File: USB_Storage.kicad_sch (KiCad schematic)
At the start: 26 parts, among them J1 USB_A, U1 USBLC6-2SC6, U2 AP2112K-3.3, U3 GL3224-ONY, U4 AP2112K-1.2, Y1 25MHz

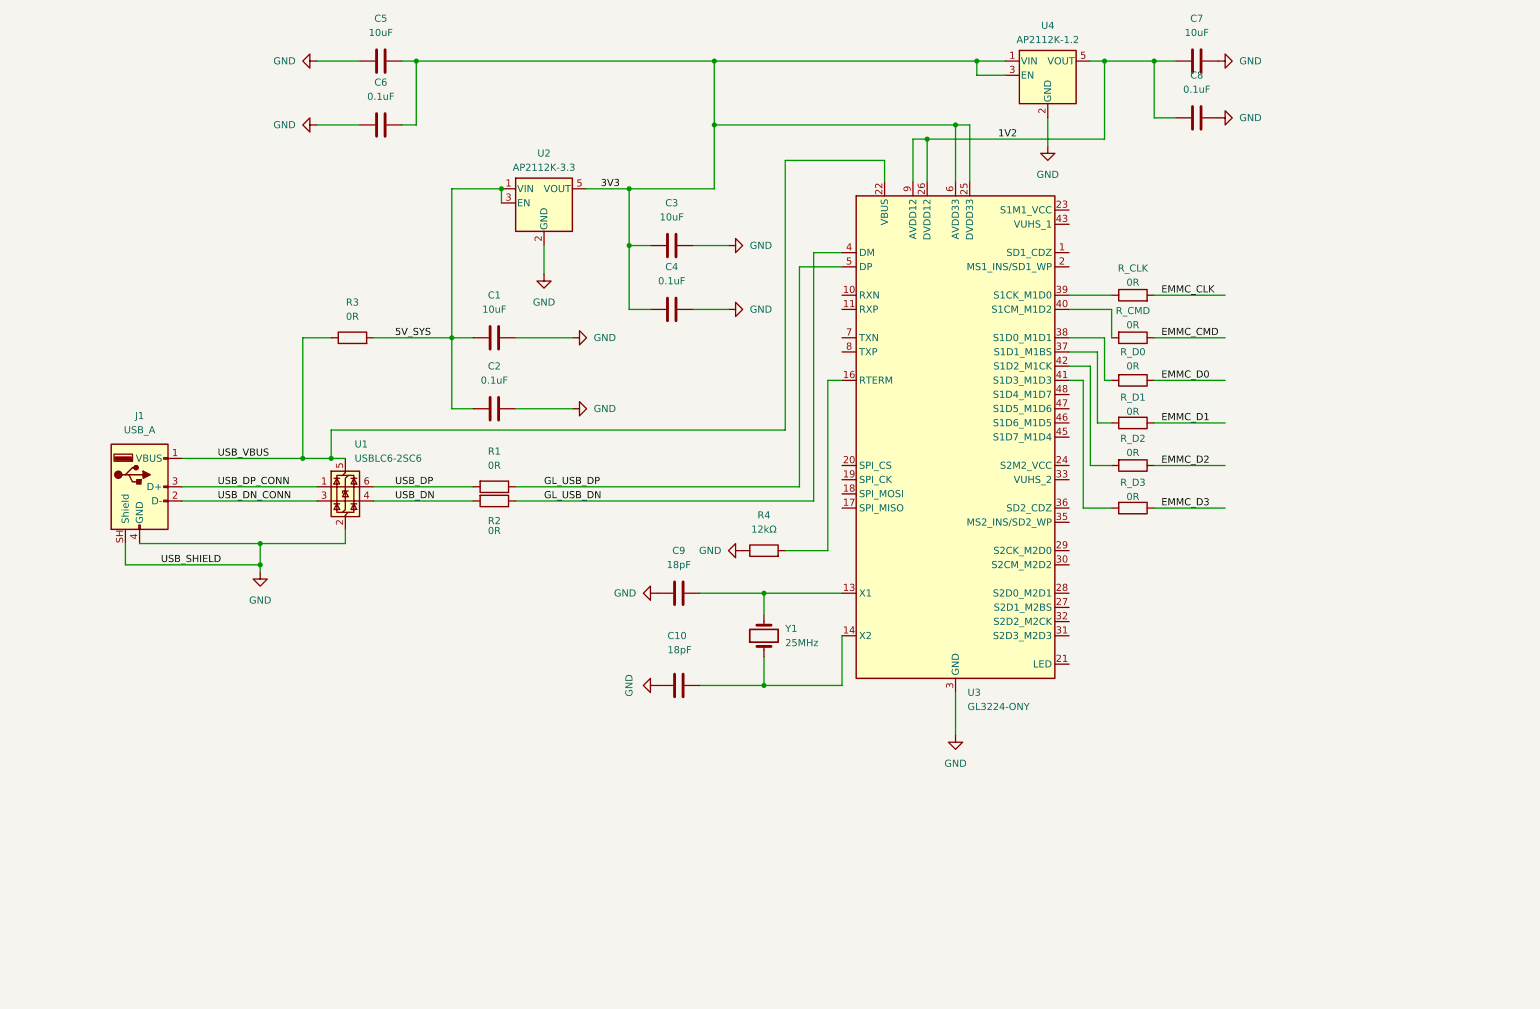
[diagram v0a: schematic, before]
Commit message: 回路図を更新しました
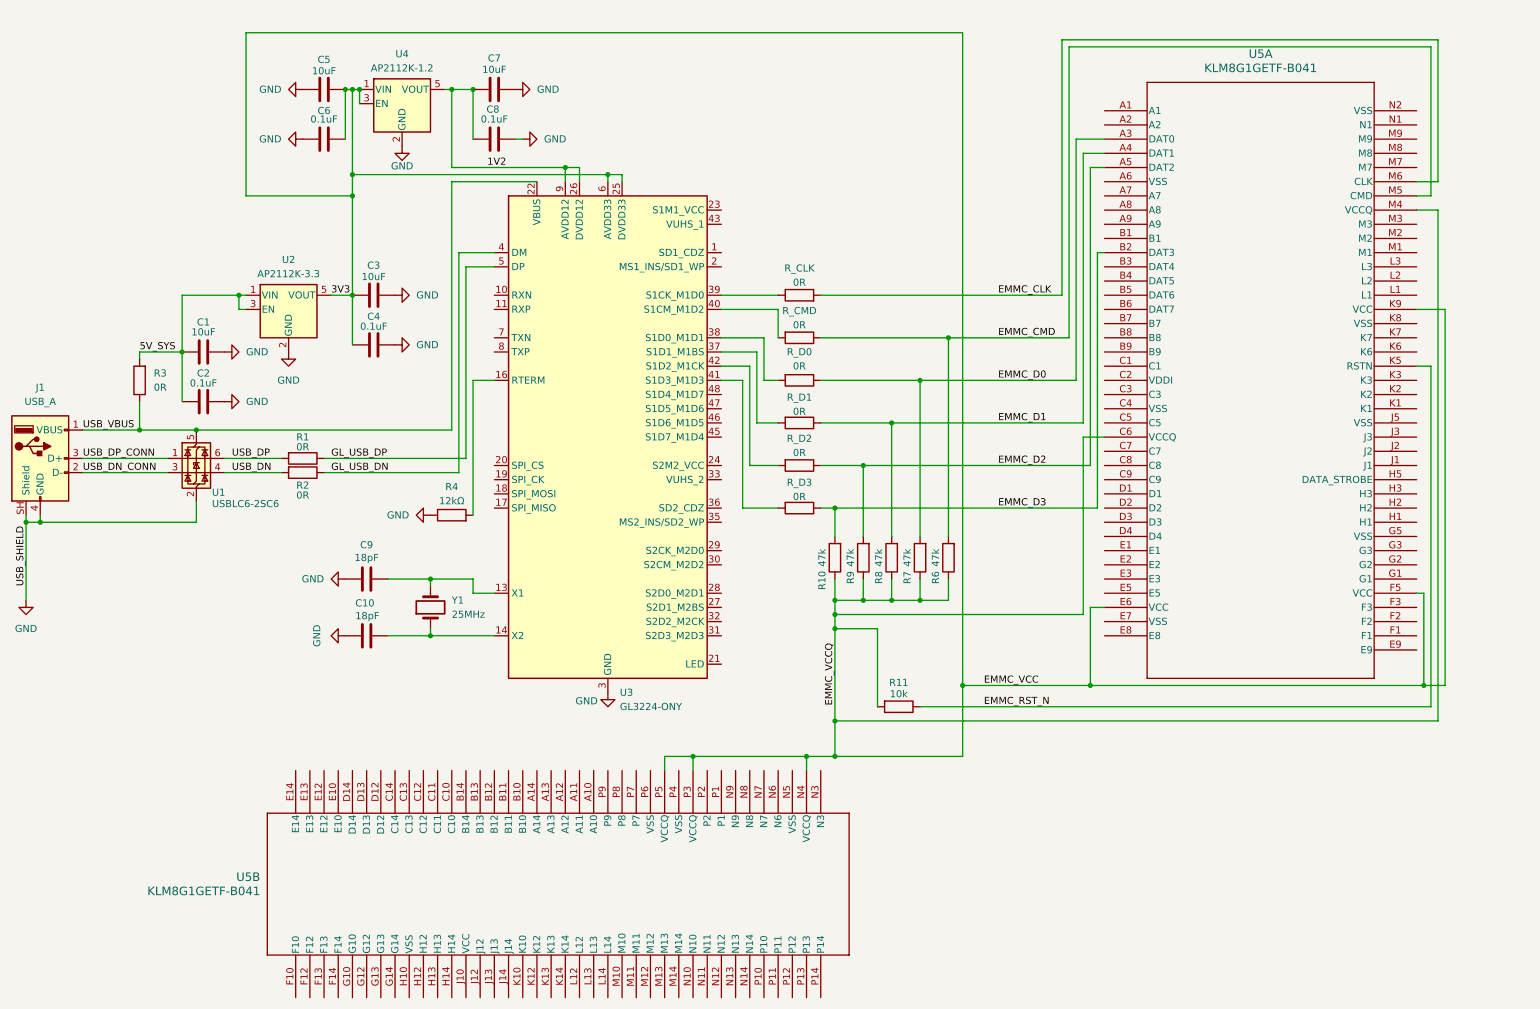
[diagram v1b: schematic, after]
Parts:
- added R10, R6, R7, R8, R9: 47k, symbol Device:R
- added R11: 10k, symbol Device:R
- added U5: KLM8G1GETF-B041, KLMBG2JENB-B041_SAM, symbol KLM8G1GETF-B041_1:KLM8G1GETF-B041
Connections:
- net 3V3: now also R10.1, R11.2, R6.1, R7.1, R8.1, R9.1, U5.C6 (VCCQ), U5.E6 (VCC), U5.F5 (VCC), U5.K9 (VCC), U5.M4 (VCCQ), U5.N4 (VCCQ), U5.P3 (VCCQ), U5.P5 (VCCQ)
- net EMMC_CLK: now also U5.M6 (CLK)
- net EMMC_CMD: now also R6.2, U5.M5 (CMD)
- net EMMC_D0: now also R7.2, U5.A3 (DAT0)
- net EMMC_D1: now also R8.2, U5.A4 (DAT1)
- net EMMC_D2: now also R9.2, U5.A5 (DAT2)
- net EMMC_D3: now also R10.2, U5.B2 (DAT3)
- new net EMMC_RST_N: R11.1, U5.K5 (RSTN)
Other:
- moved on the sheet: C1, C10, C2, C3, C4, C5, C6, C7, C8, C9, J1, R1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

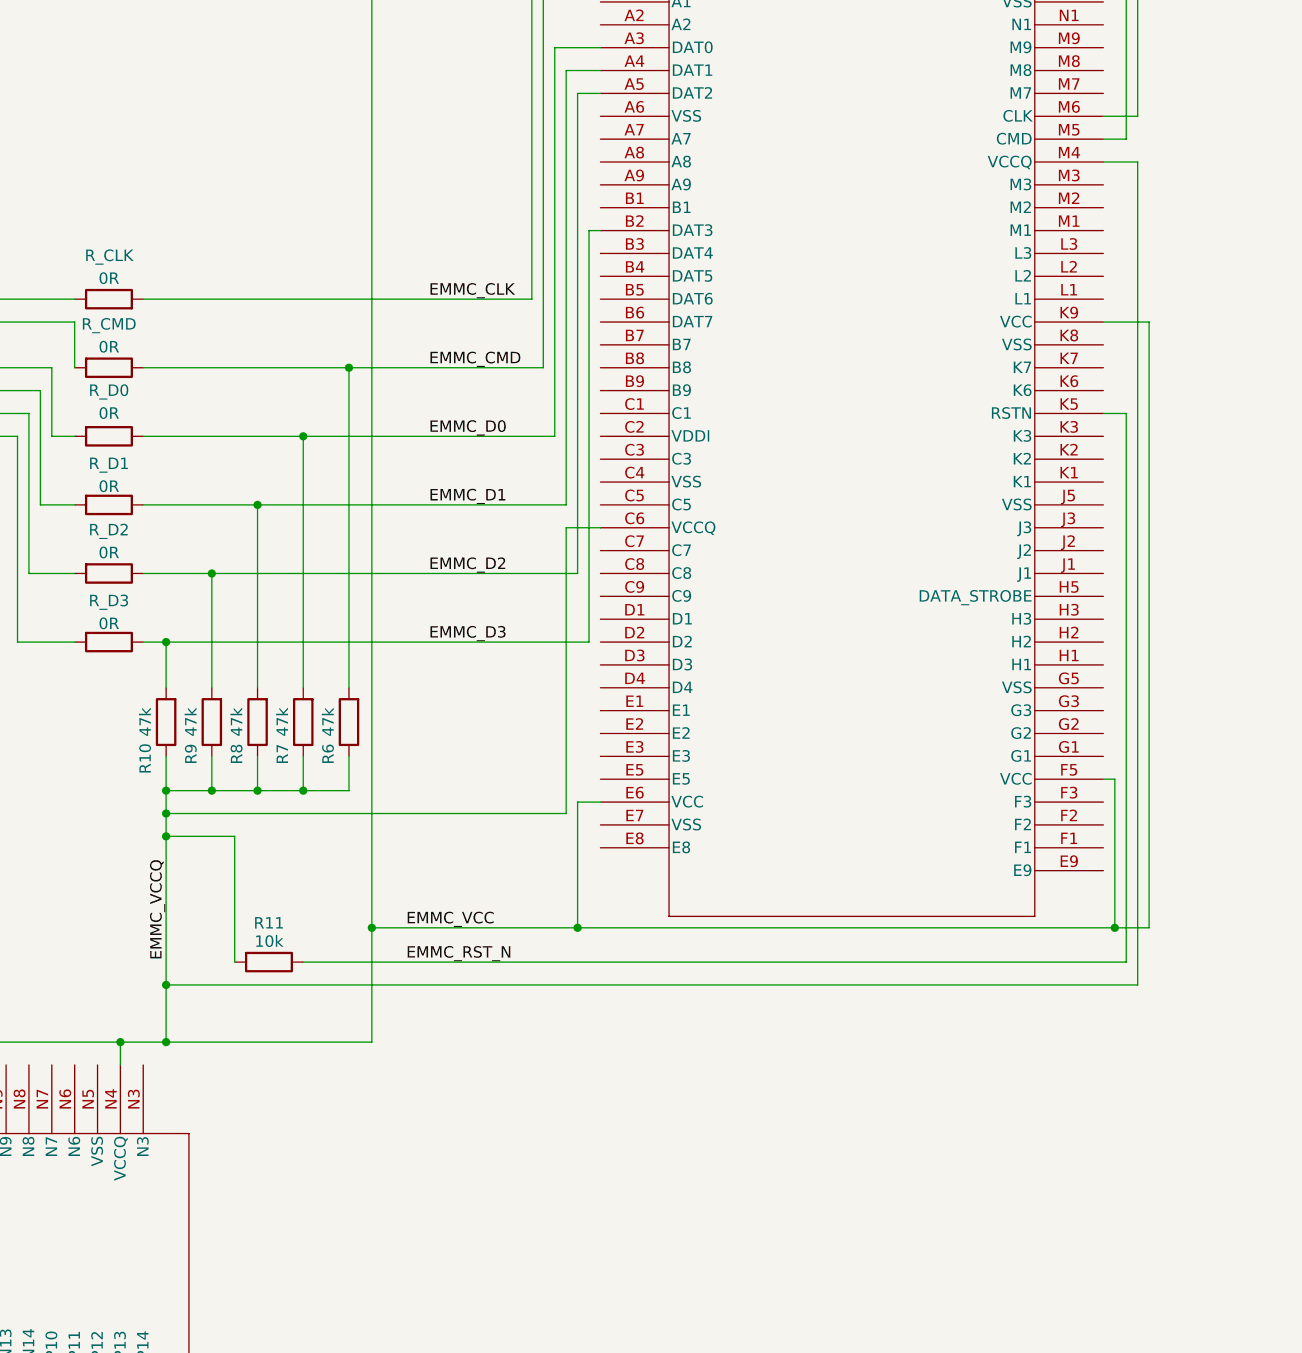
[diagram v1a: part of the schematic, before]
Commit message: 回路図の更新
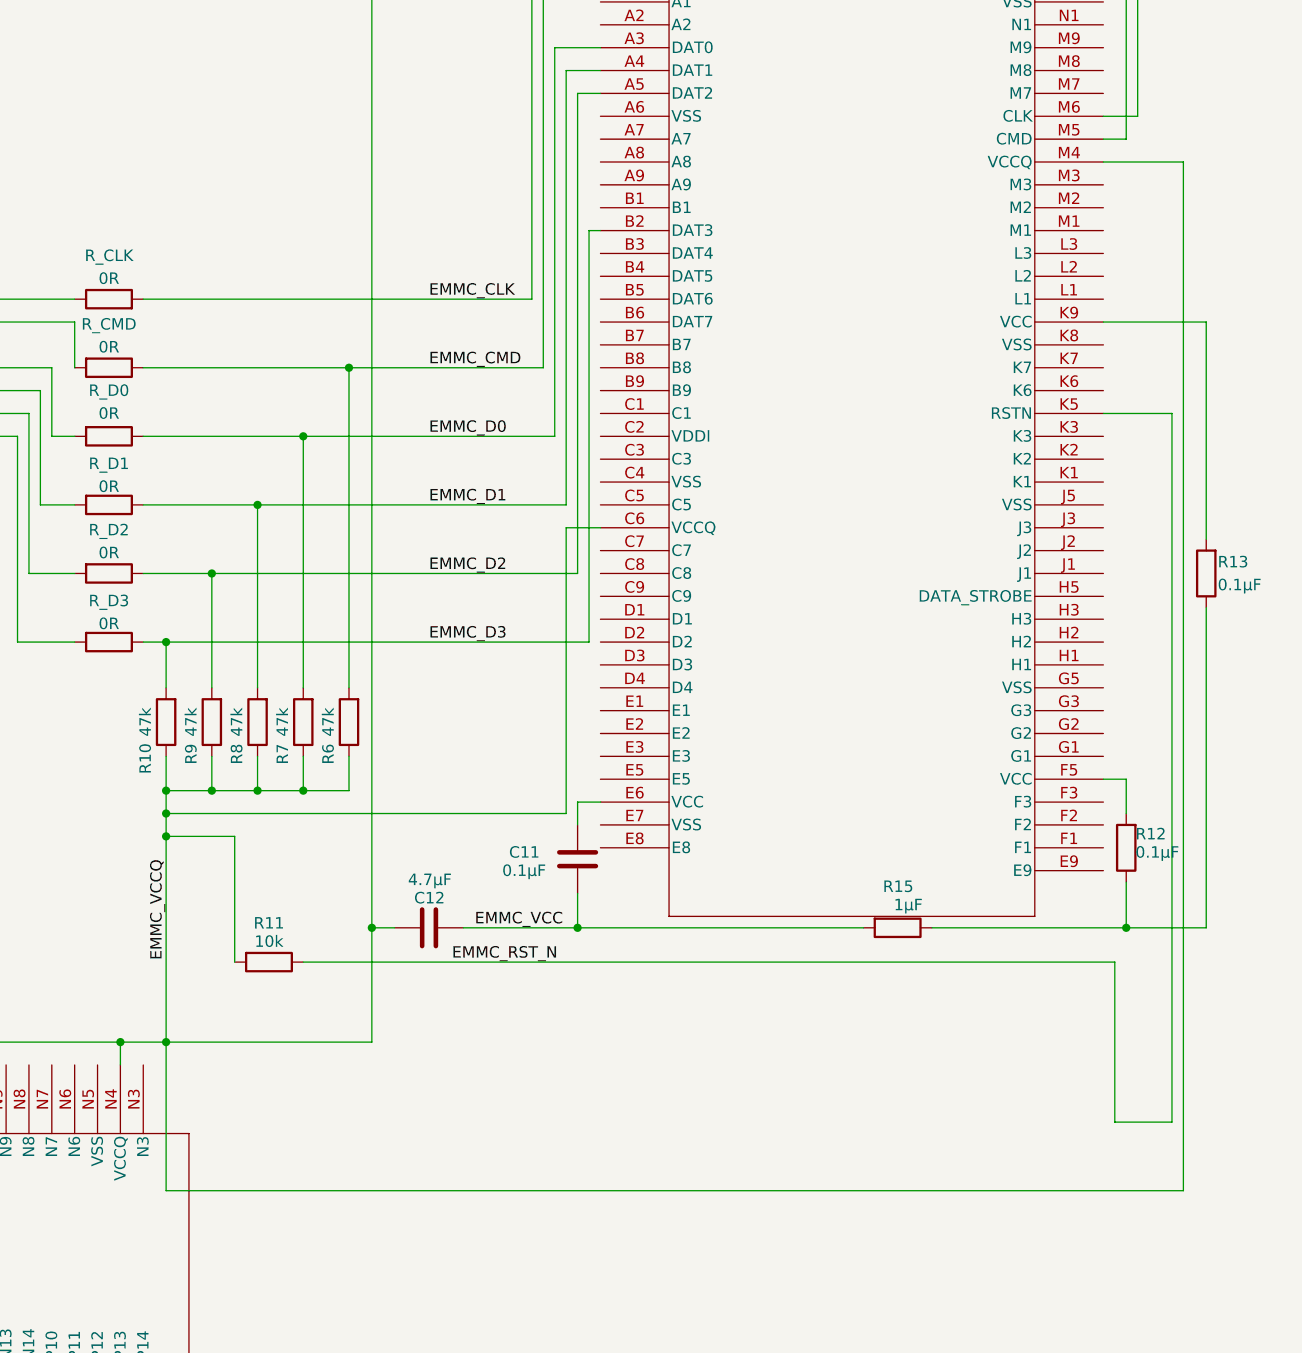
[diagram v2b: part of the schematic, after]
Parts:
- added C11: 0.1µF, symbol Device:C
- added C12: 4.7µF, symbol Device:C
- added R12, R13: 0.1µF, symbol Device:R
- added R15: 1µF, symbol Device:R
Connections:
- net 3V3: now also C12.1; no longer U5.E6 (VCC), U5.F5 (VCC), U5.K9 (VCC)
- new net: R12.1, R13.1, R15.1
- new net: R13.2, U5.K9 (VCC)
- new net: C11.1, U5.E6 (VCC)
- new net: R12.2, U5.F5 (VCC)
- new net EMMC_VCC: C11.2, C12.2, R15.2
